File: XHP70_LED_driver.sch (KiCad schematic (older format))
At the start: 24 parts, among them U1 TPS61088, U2 ATtiny816_(QFN20), U3 INA181

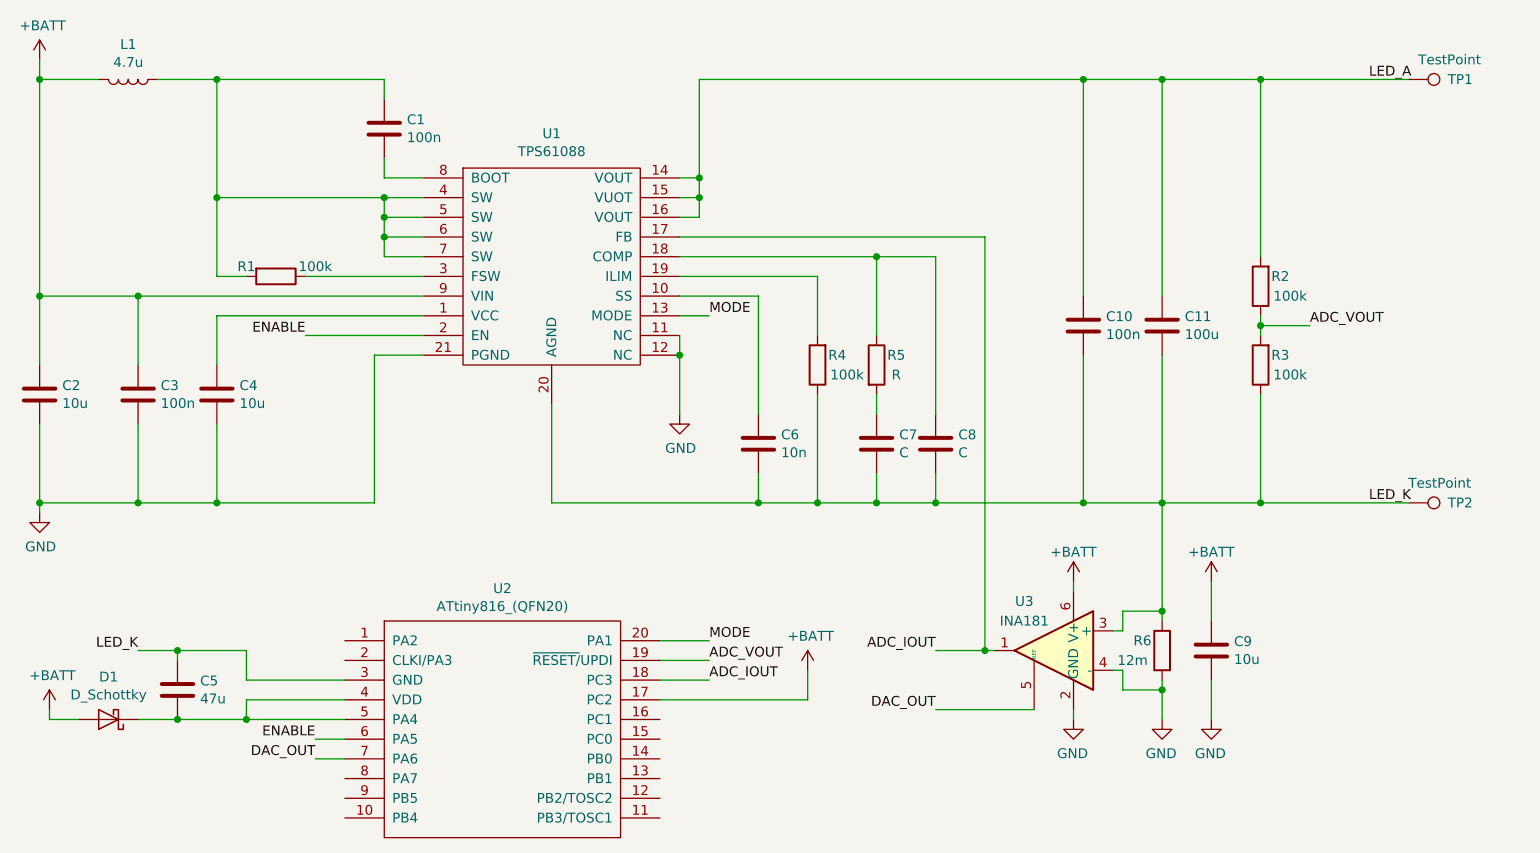
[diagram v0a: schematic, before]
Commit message: exported project milestone, fixed problems
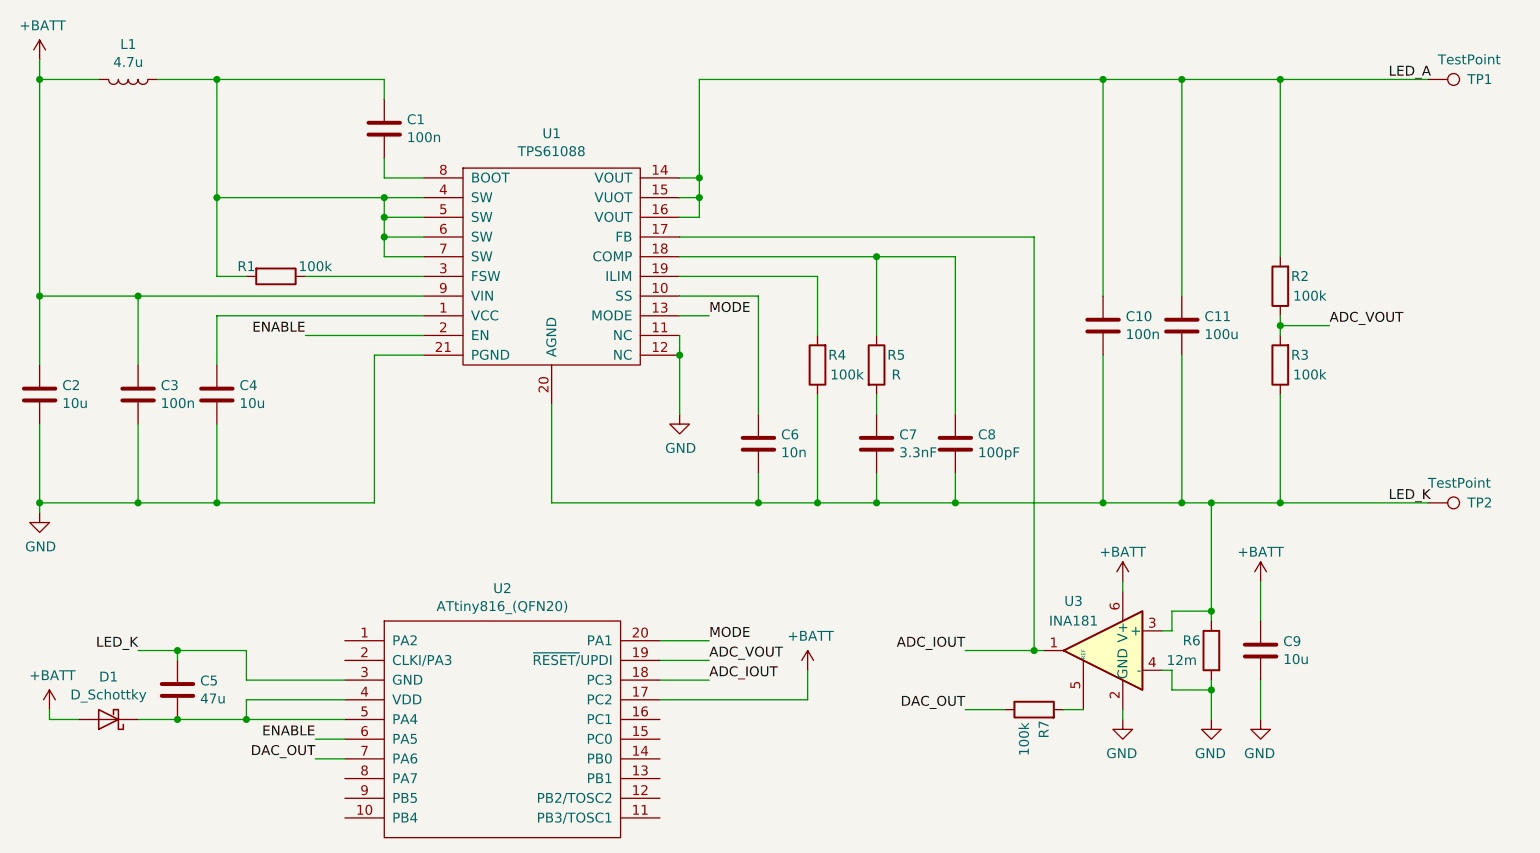
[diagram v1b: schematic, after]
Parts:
- added R7: 100k, Resistors_SMD:R_0402_NoSilk, symbol Device:R
- C7: value C -> 3.3nF
- C8: value C -> 100pF
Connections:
- net DAC_OUT: now also R7.1; no longer U3.5 (REF)
- new net: R7.2, U3.5 (REF)
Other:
- moved on the sheet: C10, C11, C8, C9, R2, R3, R6, TP1, TP2, U3
